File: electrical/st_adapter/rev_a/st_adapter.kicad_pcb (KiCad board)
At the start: 2 copper layers, 40 x 24.6 mm, 0 parts

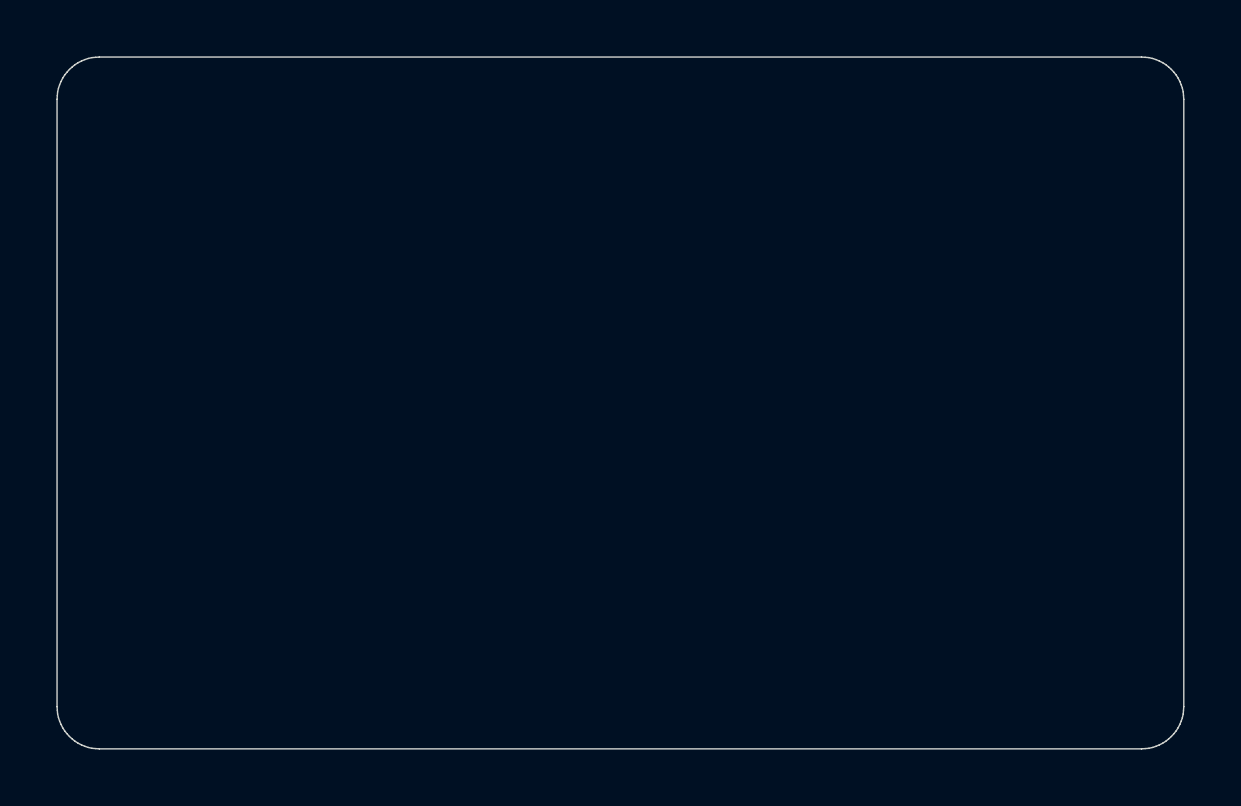
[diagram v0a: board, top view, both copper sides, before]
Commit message: Wrapped up STAdapter PCB.
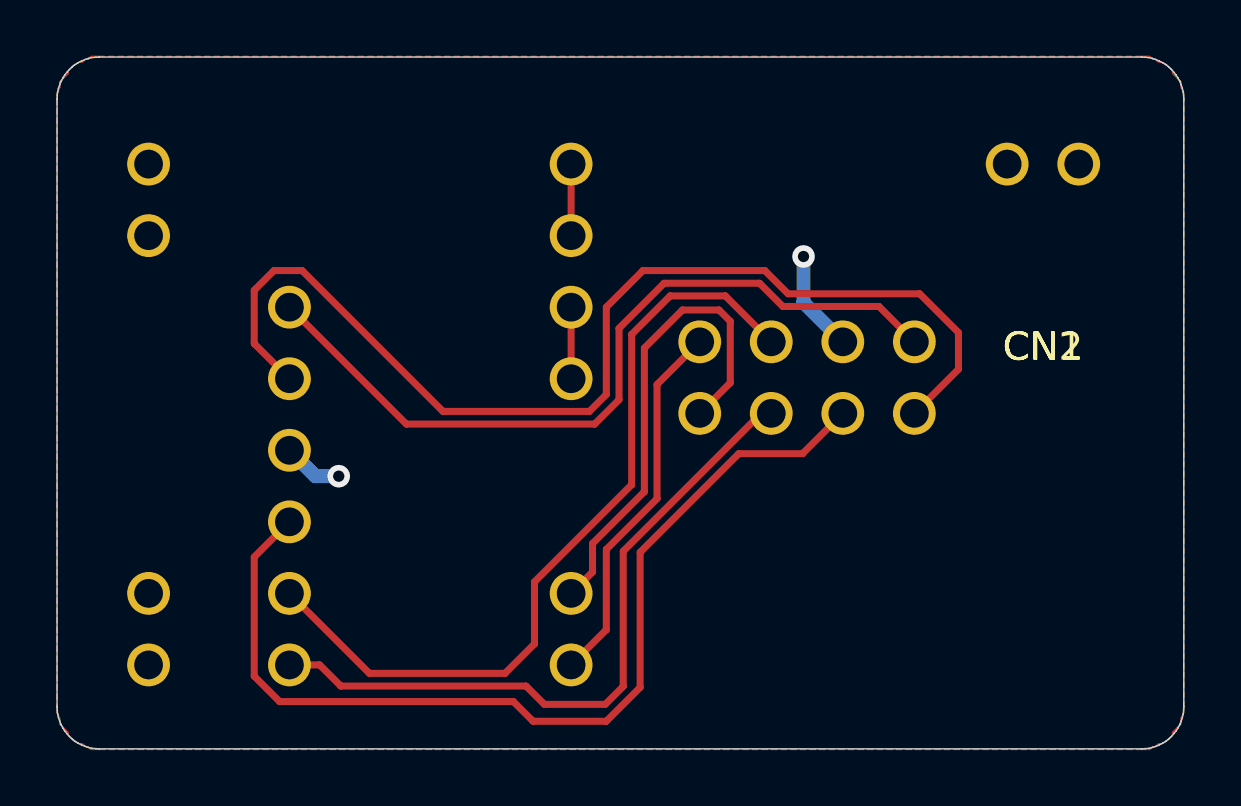
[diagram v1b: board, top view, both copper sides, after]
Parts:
- added CN1: STADAPTER;M2x4RA, HR2:STADAPTER_M2x4RA, F.Cu at (100.0, 100.0)
- added CN2: STLINK;4xF1x2+F1x4+F1x6, HR2:STADAPTER_4xF1x2+F1x4+F1x6, F.Cu at (100.0, 100.0)
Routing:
- net /SWCLK: track 0.00 -> 39.3 mm
- net /SWDIO: track 0.00 -> 34.9 mm
- net /NRST: track 0.00 -> 28.9 mm
- net /3V3: track 0.00 -> 28.3 mm
- net /SWO: track 0.00 -> 24.8 mm
- net /TX: track 0.00 -> 17.3 mm
- net /RX: track 0.00 -> 13.4 mm
- net /GND: track 0.00 -> 5.74 mm, vias 0 -> 2
- net /SWDIOX: track 0.00 -> 2.54 mm
- net /SWCLKX: track 0.00 -> 2.54 mm
- added copper zone on B.Cu, net /GND
- added copper zone on F.Cu, net /GND
